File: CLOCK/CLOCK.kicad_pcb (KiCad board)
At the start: 2 copper layers, 140 x 90 mm, 4 parts

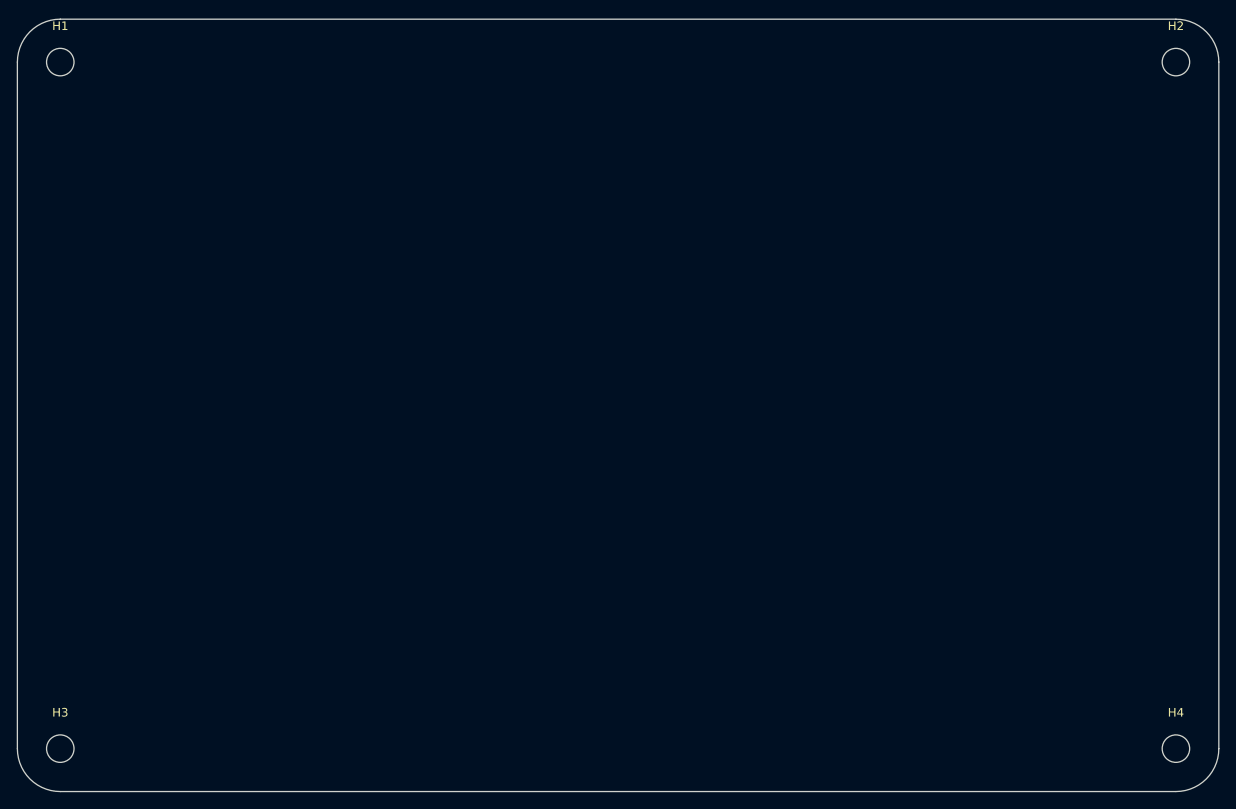
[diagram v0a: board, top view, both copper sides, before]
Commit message: WEEK4/5
PROGRSSING
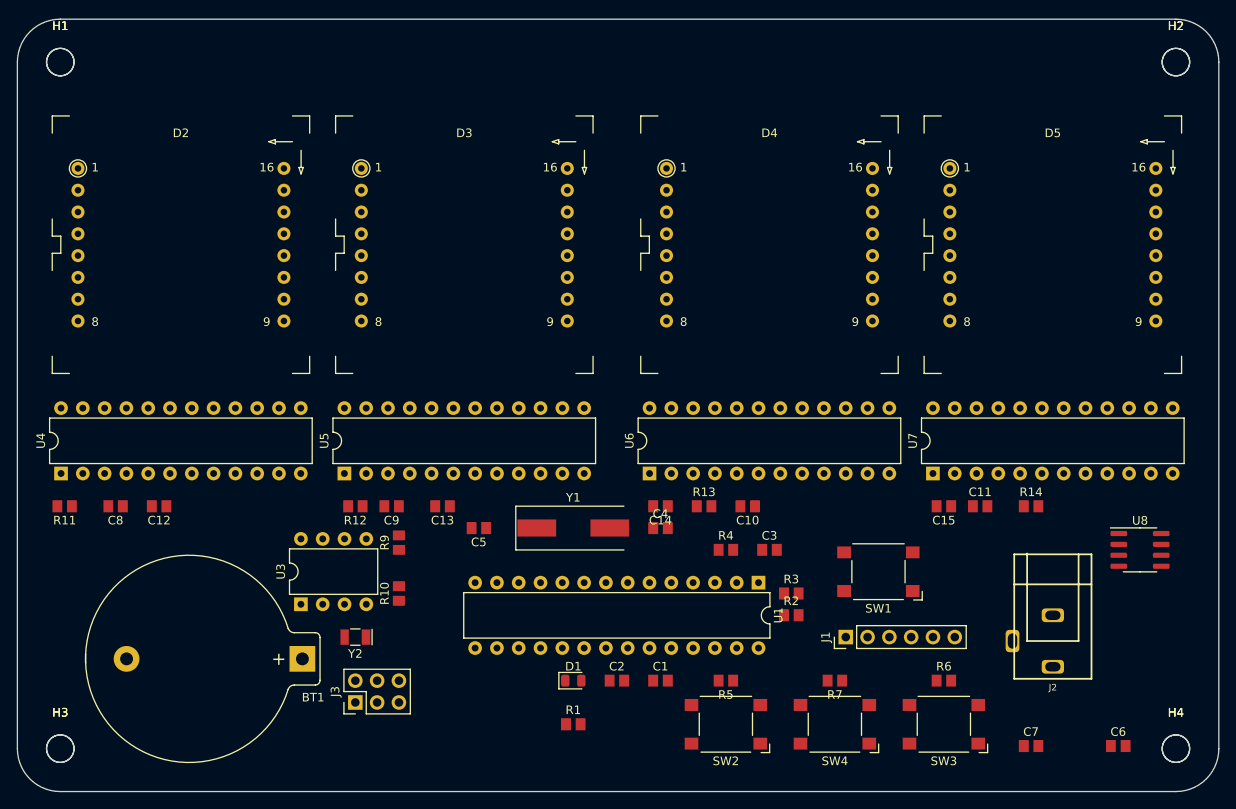
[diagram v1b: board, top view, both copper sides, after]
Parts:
- added BT1: Battery_Cell, footprints:BatteryHolder_Keystone_106_1x20mm, F.Cu at (113.2, 129.5)
- added C1: C_0805_0.1uf, footprints:C_0805_2012Metric, F.Cu at (154.9, 132.1)
- added C10: C_0805_10uf, footprints:C_0805_2012Metric, F.Cu at (165.1, 111.8)
- added C11: C_0805_10uf, footprints:C_0805_2012Metric, F.Cu at (192.2, 111.8)
- added C12: C_0805_0.1uf, footprints:C_0805_2012Metric, F.Cu at (96.5, 111.8)
- added C13: C_0805_0.1uf, footprints:C_0805_2012Metric, F.Cu at (129.5, 111.8)
- added C14: C_0805_0.1uf, footprints:C_0805_2012Metric, F.Cu at (154.9, 111.8)
- added C15: C_0805_0.1uf, footprints:C_0805_2012Metric, F.Cu at (188.0, 111.8)
- added C2: C_0805_0.1uf, footprints:C_0805_2012Metric, F.Cu at (149.9, 132.1)
- added C3: C_0805_0.1uf, footprints:C_0805_2012Metric, F.Cu at (167.6, 116.8)
- added C4: C_0805_22pf, footprints:C_0805_2012Metric, F.Cu at (154.9, 114.3)
- added C5: C_0805_22pf, footprints:C_0805_2012Metric, F.Cu at (133.8, 114.3)
- added C6: C_0805_1uf, footprints:C_0805_2012Metric, F.Cu at (208.3, 139.7)
- added C7: C_0805_0.1uf, footprints:C_0805_2012Metric, F.Cu at (198.1, 139.7)
- added C8: C_0805_10uf, footprints:C_0805_2012Metric, F.Cu at (91.4, 111.8)
- added C9: C_0805_10uf, footprints:C_0805_2012Metric, F.Cu at (123.6, 111.8)
- added D1: LED_0805, footprints:LED_0805_2012Metric, F.Cu at (144.8, 132.1)
- added D2: KWM-30881CVB, footprints:KWM-30881CVB, F.Cu at (99.1, 81.3)
- added D3: KWM-30881CVB, footprints:KWM-30881CVB, F.Cu at (132.1, 81.3)
- added D4: KWM-30881CVB, footprints:KWM-30881CVB, F.Cu at (167.6, 81.3)
- added D5: KWM-30881CVB, footprints:KWM-30881CVB, F.Cu at (200.7, 81.3)
- added H1: MountingHole, footprints:MountingHole_3.2mm_M3, F.Cu at (85.0, 60.0)
- added H2: MountingHole, footprints:MountingHole_3.2mm_M3, F.Cu at (215.0, 60.0)
- added H3: MountingHole, footprints:MountingHole_3.2mm_M3, F.Cu at (85.0, 140.0)
- added H4: MountingHole, footprints:MountingHole_3.2mm_M3, F.Cu at (215.0, 140.0)
- added J1: Conn_01x06, footprints:PinHeader_1x06_P2.54mm_Vertical, F.Cu at (176.5, 127.0)
- added J2: PJ-102AH, footprints:PJ-102AH, F.Cu at (200.7, 127.5)
- added J3: Conn_02x03_Odd_Even, footprints:PinHeader_2x03_P2.54mm_Vertical, F.Cu at (119.4, 134.6)
- added R1: R_0805_2.2K, footprints:R_0805_2012Metric, F.Cu at (144.8, 137.2)
- added R10: R_0805_4.7K, footprints:R_0805_2012Metric, F.Cu at (124.5, 121.9)
- added R11: R_0805_10K, footprints:R_0805_2012Metric, F.Cu at (85.5, 111.8)
- added R12: R_0805_10K, footprints:R_0805_2012Metric, F.Cu at (119.4, 111.8)
- added R13: R_0805_10K, footprints:R_0805_2012Metric, F.Cu at (160.0, 111.8)
- added R14: R_0805_10K, footprints:R_0805_2012Metric, F.Cu at (198.1, 111.8)
- added R2: R_0805_10K, footprints:R_0805_2012Metric, F.Cu at (170.2, 124.5)
- added R3: R_0805_47, footprints:R_0805_2012Metric, F.Cu at (170.2, 121.9)
- added R4: R_0805_47, footprints:R_0805_2012Metric, F.Cu at (162.6, 116.8)
- added R5: R_0805_10K, footprints:R_0805_2012Metric, F.Cu at (162.6, 132.1)
- added R6: R_0805_10K, footprints:R_0805_2012Metric, F.Cu at (188.0, 132.1)
- added R7: R_0805_10K, footprints:R_0805_2012Metric, F.Cu at (175.3, 132.1)
- added R9: R_0805_4.7K, footprints:R_0805_2012Metric, F.Cu at (124.5, 116.0)
- added SW1: Omron_B3F_SPST, footprints:SW_SPST_Omron_B3FS-100xP, F.Cu at (180.3, 119.4)
- added SW2: Omron_B3F_SPST, footprints:SW_SPST_Omron_B3FS-100xP, F.Cu at (162.6, 137.2)
- added SW3: Omron_B3F_SPST, footprints:SW_SPST_Omron_B3FS-100xP, F.Cu at (188.0, 137.2)
- added SW4: Omron_B3F_SPST, footprints:SW_SPST_Omron_B3FS-100xP, F.Cu at (175.3, 137.2)
- added U1: ATmega328-PU, footprints:DIP-28_W7.62mm, F.Cu at (166.4, 120.7)
- added U3: DS1307_DIP-8, footprints:DIP-8_W7.62mm, F.Cu at (113.0, 123.2)
- added U4: MAX7219, footprints:DIP-24_W7.62mm, F.Cu at (85.1, 107.9)
- added U5: MAX7219, footprints:DIP-24_W7.62mm, F.Cu at (118.1, 107.9)
- added U6: MAX7219, footprints:DIP-24_W7.62mm, F.Cu at (153.7, 107.9)
- added U7: MAX7219, footprints:DIP-24_W7.62mm, F.Cu at (186.7, 107.9)
- added U8: ADT7410, footprints:SOIC-8_3.9x4.9mm_P1.27mm, F.Cu at (210.8, 116.8)
- added Y1: Crystal_16MHz, footprints:Crystal_SMD_HC49-SD, F.Cu at (144.8, 114.3)
- added Y2: Crystal_32768Hz, footprints:Crystal_SMD_2Pin_3.2x1.5mm, F.Cu at (119.4, 127.0)
